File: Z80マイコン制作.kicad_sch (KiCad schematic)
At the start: 108 parts, among them M1 LED, SW1 SW_DIP_x08, SW2 SW_DIP_x08, SW3 SW_DIP_x08, SW4 SW_Push, SW5 SW_Push, SW6 SW_DIP_x01, SW7 SW_DIP_x08, U1 Z80CPU, U10 74HCT244, U11 74HCT244, U12 74HCT244, U13 74HCT244, U2 Z8420, U3 CY7C199, U4 74HCT244, U5 74HCT244, U6 74HCT244, U7 74HCT244, U8 74LS06N, U9 74LS06N, Y1 CXO_DIP8

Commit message: 回路図を作りました。まだ確認してません
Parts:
- removed RN4: 4.7k, Resistor_THT:R_Array_SIP9, symbol Device:R_Network08
- removed U8, U9: 74LS06N, Package_DIP:DIP-14_W7.62mm_Socket, symbol 74xx:74LS06N
- added C2, C3: 0.01u, Capacitor_THT:CP_Radial_D5.0mm_P2.00mm, symbol Device:C
- added J0, J1: Conn_01x08_Pin, Connector_PinHeader_2.54mm:PinHeader_1x08_P2.54mm_Vertical, symbol Connector:Conn_01x08_Pin
- added R39: 10k, Resistor_THT:R_Axial_DIN0204_L3.6mm_D1.6mm_P7.62mm_Horizontal, symbol Device:R
- added RN0, RN1, RN2, RN3, RN6: 4.7k, Resistor_THT:R_Array_SIP9, symbol Device:R_Network08
- added RV0: R_Potentiometer, Potentiometer_THT:Potentiometer_ACP_CA9-H5_Horizontal, symbol Device:R_Potentiometer
- added SW7: SW_Slide_DPDT, Button_Switch_THT:SW_E-Switch_EG1271_SPDT, symbol Switch:SW_Slide_DPDT
- added U13: NE555P, Package_DIP:DIP-8_W7.62mm, symbol Timer:NE555P
- A0: renamed from D7; footprint (none) -> LED_THT:LED_D3.0mm
- A1: renamed from D8; footprint (none) -> LED_THT:LED_D3.0mm
- A10: renamed from D17; footprint (none) -> LED_THT:LED_D3.0mm
- A11: renamed from D18; footprint (none) -> LED_THT:LED_D3.0mm
- A12: renamed from D21; footprint (none) -> LED_THT:LED_D3.0mm
- A13: renamed from D22; footprint (none) -> LED_THT:LED_D3.0mm
- A14: renamed from D23; footprint (none) -> LED_THT:LED_D3.0mm
- A2: renamed from D9; footprint (none) -> LED_THT:LED_D3.0mm
- A3: renamed from D10; footprint (none) -> LED_THT:LED_D3.0mm
- A4: renamed from D11; footprint (none) -> LED_THT:LED_D3.0mm
- A5: renamed from D12; footprint (none) -> LED_THT:LED_D3.0mm
- A6: renamed from D13; footprint (none) -> LED_THT:LED_D3.0mm
- A7: renamed from D14; footprint (none) -> LED_THT:LED_D3.0mm
- A8: renamed from D15; footprint (none) -> LED_THT:LED_D3.0mm
- A9: renamed from D16; footprint (none) -> LED_THT:LED_D3.0mm
- C1: renamed from C2; value 10u -> 100u
- CLK0: renamed from CLK; footprint (none) -> LED_THT:LED_D3.0mm
- D0: renamed from D25; footprint (none) -> LED_THT:LED_D3.0mm
- D1: renamed from D26; footprint (none) -> LED_THT:LED_D3.0mm
- D2: renamed from D27; footprint (none) -> LED_THT:LED_D3.0mm
- D3: renamed from D28; footprint (none) -> LED_THT:LED_D3.0mm
- D4: renamed from D29; footprint (none) -> LED_THT:LED_D3.0mm
- D5: renamed from D30; footprint (none) -> LED_THT:LED_D3.0mm
- D6: renamed from D31; footprint (none) -> LED_THT:LED_D3.0mm
- D7: renamed from D32; footprint (none) -> LED_THT:LED_D3.0mm
- D8: renamed from D40; footprint (none) -> LED_THT:LED_D3.0mm
- IORQ0: renamed from IORQ; footprint (none) -> LED_THT:LED_D3.0mm
- M0: renamed from M1; footprint (none) -> LED_THT:LED_D3.0mm
- MREQ0: renamed from MREQ; footprint (none) -> LED_THT:LED_D3.0mm
- R0: renamed from R9; footprint (none) -> Resistor_THT:R_Axial_DIN0204_L3.6mm_D1.6mm_P7.62mm_Horizontal
- R1: renamed from R10; footprint (none) -> Resistor_THT:R_Axial_DIN0204_L3.6mm_D1.6mm_P7.62mm_Horizontal
- R10: renamed from R19; footprint (none) -> Resistor_THT:R_Axial_DIN0204_L3.6mm_D1.6mm_P7.62mm_Horizontal
- R11: renamed from R20; footprint (none) -> Resistor_THT:R_Axial_DIN0204_L3.6mm_D1.6mm_P7.62mm_Horizontal
- R12: renamed from R21; footprint (none) -> Resistor_THT:R_Axial_DIN0204_L3.6mm_D1.6mm_P7.62mm_Horizontal
- R13: renamed from R22; footprint (none) -> Resistor_THT:R_Axial_DIN0204_L3.6mm_D1.6mm_P7.62mm_Horizontal
- R14: renamed from R23; footprint (none) -> Resistor_THT:R_Axial_DIN0204_L3.6mm_D1.6mm_P7.62mm_Horizontal
- R15: renamed from R25; footprint (none) -> Resistor_THT:R_Axial_DIN0204_L3.6mm_D1.6mm_P7.62mm_Horizontal
- R16: renamed from R26; footprint (none) -> Resistor_THT:R_Axial_DIN0204_L3.6mm_D1.6mm_P7.62mm_Horizontal
- R17: renamed from R27; footprint (none) -> Resistor_THT:R_Axial_DIN0204_L3.6mm_D1.6mm_P7.62mm_Horizontal
- R18: renamed from R28; footprint (none) -> Resistor_THT:R_Axial_DIN0204_L3.6mm_D1.6mm_P7.62mm_Horizontal
- R19: renamed from R29; footprint (none) -> Resistor_THT:R_Axial_DIN0204_L3.6mm_D1.6mm_P7.62mm_Horizontal
- R2: renamed from R11; footprint (none) -> Resistor_THT:R_Axial_DIN0204_L3.6mm_D1.6mm_P7.62mm_Horizontal
- R20: renamed from R30; footprint (none) -> Resistor_THT:R_Axial_DIN0204_L3.6mm_D1.6mm_P7.62mm_Horizontal
- R21: renamed from R31; footprint (none) -> Resistor_THT:R_Axial_DIN0204_L3.6mm_D1.6mm_P7.62mm_Horizontal
- R22: renamed from R32; footprint (none) -> Resistor_THT:R_Axial_DIN0204_L3.6mm_D1.6mm_P7.62mm_Horizontal
- R23: renamed from R33; footprint (none) -> Resistor_THT:R_Axial_DIN0204_L3.6mm_D1.6mm_P7.62mm_Horizontal
- R24: renamed from R34; footprint (none) -> Resistor_THT:R_Axial_DIN0204_L3.6mm_D1.6mm_P7.62mm_Horizontal
- R25: renamed from R35; footprint (none) -> Resistor_THT:R_Axial_DIN0204_L3.6mm_D1.6mm_P7.62mm_Horizontal
- R26: renamed from R36; footprint (none) -> Resistor_THT:R_Axial_DIN0204_L3.6mm_D1.6mm_P7.62mm_Horizontal
- R27: renamed from R37; footprint (none) -> Resistor_THT:R_Axial_DIN0204_L3.6mm_D1.6mm_P7.62mm_Horizontal
- R28: renamed from R38; footprint (none) -> Resistor_THT:R_Axial_DIN0204_L3.6mm_D1.6mm_P7.62mm_Horizontal
- R29: renamed from R39; footprint (none) -> Resistor_THT:R_Axial_DIN0204_L3.6mm_D1.6mm_P7.62mm_Horizontal
- R3: renamed from R12; footprint (none) -> Resistor_THT:R_Axial_DIN0204_L3.6mm_D1.6mm_P7.62mm_Horizontal
- R30: renamed from R40; footprint (none) -> Resistor_THT:R_Axial_DIN0204_L3.6mm_D1.6mm_P7.62mm_Horizontal
- R31: renamed from R8; footprint (none) -> Resistor_THT:R_Axial_DIN0204_L3.6mm_D1.6mm_P7.62mm_Horizontal
- R4: renamed from R13; footprint (none) -> Resistor_THT:R_Axial_DIN0204_L3.6mm_D1.6mm_P7.62mm_Horizontal
- R5: renamed from R14; footprint (none) -> Resistor_THT:R_Axial_DIN0204_L3.6mm_D1.6mm_P7.62mm_Horizontal
- R6: renamed from R15; footprint (none) -> Resistor_THT:R_Axial_DIN0204_L3.6mm_D1.6mm_P7.62mm_Horizontal
- R7: renamed from R16; footprint (none) -> Resistor_THT:R_Axial_DIN0204_L3.6mm_D1.6mm_P7.62mm_Horizontal
- R8: renamed from R17; footprint (none) -> Resistor_THT:R_Axial_DIN0204_L3.6mm_D1.6mm_P7.62mm_Horizontal
- R9: renamed from R18; footprint (none) -> Resistor_THT:R_Axial_DIN0204_L3.6mm_D1.6mm_P7.62mm_Horizontal
- RD0: renamed from RD; footprint (none) -> LED_THT:LED_D3.0mm
- WAIT0: renamed from WAIT; footprint (none) -> LED_THT:LED_D3.0mm
- WR0: renamed from WR; footprint (none) -> LED_THT:LED_D3.0mm
- renumbered SW2 to A0-A7, SW7 to A8-A14, C1 to C0, SW3 to D0-D7, SW1 to I0-I7, D1 to O0, D2 to O1, D3 to O2, D4 to O3, D5 to O4, D6 to O5, D19 to O6, D20 to O7, R3 to R32, R4 to R33, R5 to R34, R7 to R35, R6 to R36, R1 to R37, R2 to R38, RN3 to RN4, RN1 to RN5, RN5 to RN7, RN2 to RN8, SW5 to SW0, SW6 to SW1, TP1 to TP0, TP2 to TP1, U7 to U0, U10 to U1, U6 to U10, U12 to U2, U13 to U3, U1 to U4, U2 to U5, U3 to U6, U4 to U8, U5 to U9, SW4 to WRITE0, Y1 to Y0
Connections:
- net GND: now also A0-A7.1, A0-A7.2, A0-A7.3, A0-A7.4, A0-A7.5, A0-A7.6, A0-A7.7, A0-A7.8, O0.1 (K), O1.1 (K), O2.1 (K), O3.1 (K), O4.1 (K), O5.1 (K), O6.1 (K), O7.1 (K), RN5.2 (R1), RN5.3 (R2), RN5.4 (R3), RN5.5 (R4), RN5.6 (R5), RN5.7 (R6), RN5.8 (R7), RN5.9 (R8), U11.11 (2A3), U11.13 (2A2), U11.15 (2A1), U11.17 (2A0), U11.2 (1A0), U11.4 (1A1), U11.6 (1A2), U11.8 (1A3), SW7.5 (B); no longer Y0.4 (GND)
- net VCC: now also RN8.1 (common), R39.1, RN0.1 (common), RN1.1 (common), RN2.1 (common), RN3.1 (common), RN6.1 (common), U13.4 (R), U13.8 (VCC); no longer D0-D7.6, RN8.4 (R3), U8.15 (2A1)
- net at I0-I7.1, RN7.2 (R1), U5.15 (PA0): now also J1.8 (Pin_8)
- net at I0-I7.2, RN7.3 (R2), U5.14 (PA1): now also J1.7 (Pin_7)
- net at I0-I7.3, RN7.4 (R3), U5.13 (PA2): now also J1.6 (Pin_6)
- net at I0-I7.4, RN7.5 (R4), U5.12 (PA3): now also J1.5 (Pin_5)
- net at I0-I7.5, RN7.6 (R5), U5.10 (PA4): now also J1.4 (Pin_4)
- net at I0-I7.6, RN7.7 (R6), U5.9 (PA5): now also J1.3 (Pin_3)
- net at I0-I7.7, RN7.8 (R7), U5.8 (PA6): now also J1.2 (Pin_2)
- net at I0-I7.8, RN7.9 (R8), U5.7 (PA7): now also J1.1 (Pin_1)
- net at U10.1 (1OE), U10.19 (2OE), U11.1 (1OE)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: now also RN0.9 (R8)
- net at U10.14 (1Y2), U3.15 (2A1), U4.19 (~{MREQ})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: now also RN0.7 (R6)
- net at U10.16 (1Y1), U3.17 (2A0), U4.22 (~{WR})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: now also RN0.6 (R5)
- net at U10.18 (1Y0), U3.8 (1A3), U4.21 (~{RD})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: now also RN0.5 (R4)
- net at O3.2 (A): now also U5.31 (PB4), J0.4 (Pin_4), RN6.6 (R5)
- net at U1.8 (1A3), U4.1 (A11), U6.7 (A11)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: now also RN2.5 (R4)
- net at U1.6 (1A2), U4.40 (A10), U6.6 (A10)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: now also RN2.4 (R3)
- net at U1.4 (1A1), U4.39 (A9), U6.5 (A9)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: now also RN2.3 (R2)
- net at U1.2 (1A0), U4.38 (A8), U6.4 (A8)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: now also RN2.2 (R1)
- net at U1.17 (2A0), U4.2 (A12), U6.8 (A12)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: now also RN2.6 (R5)
- net at U1.15 (2A1), U4.3 (A13), U6.9 (A13)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: now also RN2.7 (R6)
- net at U1.13 (2A2), U4.4 (A14), U6.10 (A14)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: now also RN2.8 (R7)
- net at U2.8 (1A3), U4.8 (D3), U5.40 (D3)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: now also RN1.5 (R4)
- net at U2.6 (1A2), U4.12 (D2), U5.1 (D2)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: now also RN1.4 (R3)
- net at U2.4 (1A1), U4.15 (D1), U5.20 (D1)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: now also RN1.3 (R2)
- net at U2.2 (1A0), U4.14 (D0), U5.19 (D0)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: now also RN1.2 (R1)
- net at U2.17 (2A0), U4.7 (D4), U5.39 (D4)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: now also RN1.6 (R5)
- net at U2.15 (2A1), U4.9 (D5), U5.38 (D5)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: now also RN1.7 (R6)
- net at U2.13 (2A2), U4.10 (D6), U5.3 (D6)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: now also RN1.8 (R7)
- net at U2.11 (2A3), U4.13 (D7), U5.2 (D7)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: now also RN1.9 (R8)
- net at O4.2 (A): now also U5.30 (PB3), J0.5 (Pin_5), RN6.5 (R4)
- net at O5.2 (A): now also U5.29 (PB2), J0.6 (Pin_6), RN6.4 (R3)
- net at U5.27 (PB0): now also O7.2 (A), J0.8 (Pin_8), RN6.2 (R1)
- net at O0.2 (A): now also U5.34 (PB7), J0.1 (Pin_1), RN6.9 (R8)
- net at U0.11 (2A3), U11.9 (2Y3), U4.37 (A7)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: now also RN3.9 (R8)
- net at U0.13 (2A2), U11.7 (2Y2), U4.36 (A6)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: now also RN3.8 (R7)
- net at U0.15 (2A1), U11.5 (2Y1), U4.35 (A5)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: now also RN3.7 (R6)
- net at U0.17 (2A0), U11.3 (2Y0), U4.34 (A4)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: now also RN3.6 (R5)
- net at U0.2 (1A0), U11.18 (1Y0), U4.30 (A0)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: now also RN3.2 (R1)
- net at U0.4 (1A1), U11.16 (1Y1), U4.31 (A1)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: now also RN3.3 (R2)
- net at U0.6 (1A2), U11.14 (1Y2), U4.32 (A2)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: now also RN3.4 (R3)
- net at U0.8 (1A3), U11.12 (1Y3), U4.33 (A3)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: now also RN3.5 (R4)
- net at U3.2 (1A0), U4.6 (~{CLK}), U5.25 (CLK): now also RN0.2 (R1), SW7.2 (B); no longer R35.1, Y0.5 (OUT)
- net at U5.33 (PB6): now also O1.2 (A), J0.2 (Pin_2), RN6.8 (R7)
- net at U5.28 (PB1): now also O6.2 (A), J0.7 (Pin_7), RN6.3 (R2)
- net at O2.2 (A): now also U5.32 (PB5), J0.3 (Pin_3), RN6.7 (R6)
- net at U3.13 (2A2), U4.20 (~{IORQ}), U5.36 (~{IORQ})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: now also RN0.8 (R7)
- net at U3.4 (1A1), U4.27 (~{M1}), U5.37 (~{M1}): now also RN0.3 (R2)
- net at R34.2, U3.6 (1A2), U4.17 (~{NMI})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: now also RN0.4 (R3)
- new net: C2.2, C3.2, U13.1 (GND)
- new net: C3.1, RV0.2, U13.2 (TR), U13.6 (THR)
- new net: SW7.3 (C), U13.3 (Q)
- new net: C2.1, SW7.4 (A), U13.5 (CV)
- new net: R39.2, RV0.3, U13.7 (DIS)
- new net: D0-D7.6, RN8.4 (R3), U8.15 (2A1)
- new net: R35.1, SW7.1 (A), Y0.5 (OUT)
- new net: SW7.6 (C), Y0.4 (GND)
- no-connect marks 31 -> 27
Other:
- moved on the sheet: A0, A0-A7, A1, A10, A11, A12, A13, A14, A2, A3, A4, A5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

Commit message: 基盤確認済み、PCBに入りました
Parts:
- added R40: 4.7k, Resistor_THT:R_Axial_DIN0204_L3.6mm_D1.6mm_P7.62mm_Horizontal, symbol Device:R
- added U7: 74HCT244, Package_DIP:DIP-20_W7.62mm_Socket, symbol 74xx:74HCT244
- renumbered D8 to BUSACK0, SW0 to RESET0
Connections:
- net GND: no longer A0-A7.1, A0-A7.2, A0-A7.3, A0-A7.4, A0-A7.5, A0-A7.6, A0-A7.7, A0-A7.8, RN5.2 (R1), RN5.3 (R2), RN5.4 (R3), RN5.5 (R4), RN5.6 (R5), RN5.7 (R6), RN5.8 (R7), RN5.9 (R8), U11.11 (2A3), U11.13 (2A2), U11.15 (2A1), U11.17 (2A0), U11.2 (1A0), U11.4 (1A1), U11.6 (1A2), U11.8 (1A3)
- net VCC: now also R40.1
- net at J0.4 (Pin_4), O3.2 (A), RN6.6 (R5): now also U7.3 (2Y0); no longer U5.31 (PB4)
- net at J0.1 (Pin_1), O0.2 (A), RN6.9 (R8): now also U7.9 (2Y3); no longer U5.34 (PB7)
- net at J0.2 (Pin_2), O1.2 (A), RN6.8 (R7): now also U7.7 (2Y2); no longer U5.33 (PB6)
- net at J0.3 (Pin_3), O2.2 (A), RN6.7 (R6): now also U7.5 (2Y1); no longer U5.32 (PB5)
- net at J0.5 (Pin_5), O4.2 (A), RN6.5 (R4): now also U7.12 (1Y3); no longer U5.30 (PB3)
- net at J0.6 (Pin_6), O5.2 (A), RN6.4 (R3): now also U7.14 (1Y2); no longer U5.29 (PB2)
- net at J0.7 (Pin_7), O6.2 (A), RN6.3 (R2): now also U7.16 (1Y1); no longer U5.28 (PB1)
- net at J0.8 (Pin_8), O7.2 (A), RN6.2 (R1): now also U7.18 (1Y0); no longer U5.27 (PB0)
- new net: A0-A7.1, RN5.2 (R1), U11.2 (1A0)
- new net: A0-A7.2, RN5.3 (R2), U11.4 (1A1)
- new net: A0-A7.3, RN5.4 (R3), U11.6 (1A2)
- new net: A0-A7.4, RN5.5 (R4), U11.8 (1A3)
- new net: A0-A7.5, RN5.6 (R5), U11.17 (2A0)
- new net: A0-A7.6, RN5.7 (R6), U11.15 (2A1)
- new net: A0-A7.7, RN5.8 (R7), U11.13 (2A2)
- new net: A0-A7.8, RN5.9 (R8), U11.11 (2A3)
- new net: R40.2, U7.1 (1OE), U7.19 (2OE)
- new net: U5.34 (PB7), U7.11 (2A3)
- new net: U5.33 (PB6), U7.13 (2A2)
- new net: U5.32 (PB5), U7.15 (2A1)
- new net: U5.31 (PB4), U7.17 (2A0)
- new net: U5.27 (PB0), U7.2 (1A0)
- new net: U5.28 (PB1), U7.4 (1A1)
- new net: U5.29 (PB2), U7.6 (1A2)
- new net: U5.30 (PB3), U7.8 (1A3)
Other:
- moved on the sheet: D0-D7, I0-I7, J0, J1, O0, O1, O2, O3, O4, O5, O6, O7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

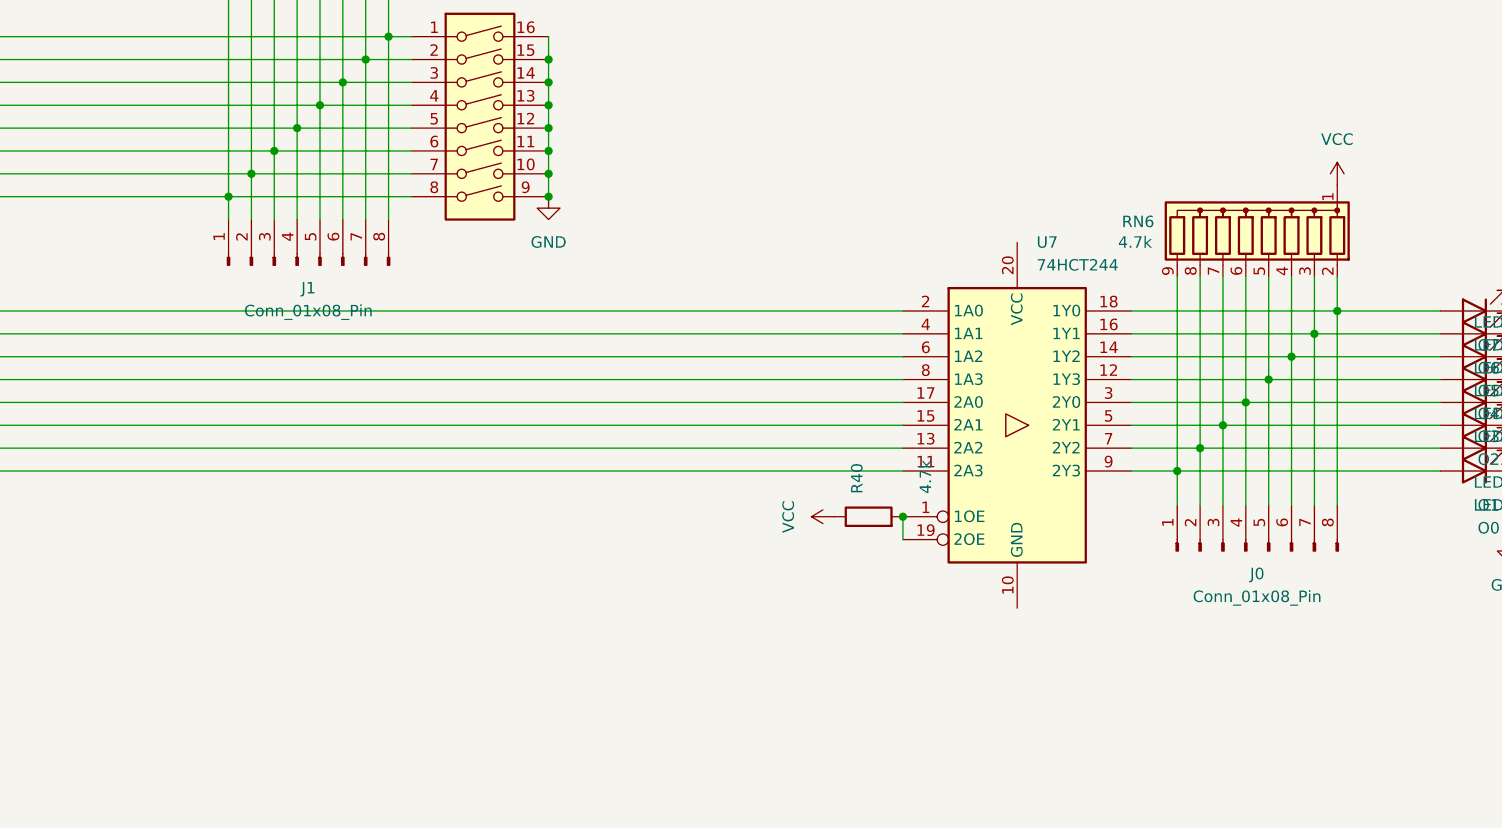
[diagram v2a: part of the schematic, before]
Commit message: 基盤のVCC,GND配線終わりました
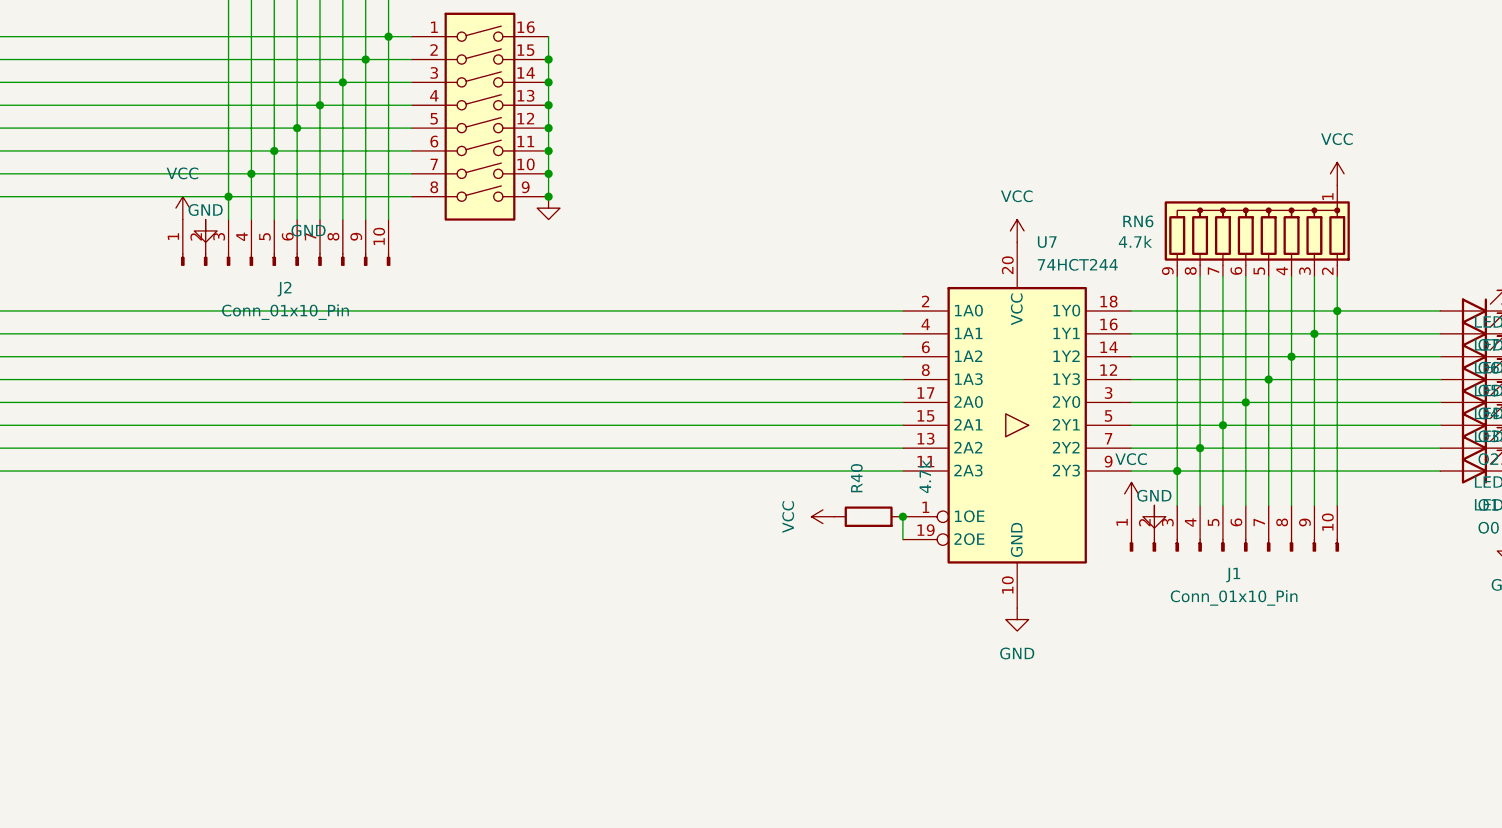
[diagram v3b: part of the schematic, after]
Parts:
- removed J0, J1: Conn_01x08_Pin, Connector_PinHeader_2.54mm:PinHeader_1x08_P2.54mm_Vertical, symbol Connector:Conn_01x08_Pin
- added J1, J2: Conn_01x10_Pin, Connector_PinHeader_2.54mm:PinHeader_1x10_P2.54mm_Vertical, symbol Connector:Conn_01x10_Pin
- A0-A7, A8-A14, D0-D7, I0-I7: footprint Package_DIP:CERDIP-16_W7.62mm_SideBrazed_Socket -> Package_DIP:DIP-16_W7.62mm_Socket
- U13: footprint Package_DIP:DIP-8_W7.62mm -> Package_DIP:DIP-8_W7.62mm_Socket
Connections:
- net GND: now also U7.10 (GND), J1.2 (Pin_2), J2.2 (Pin_2)
- net VCC: now also U7.20 (VCC), J1.1 (Pin_1), J2.1 (Pin_1)
- net at I0-I7.1, RN7.2 (R1), U5.15 (PA0): now also J2.10 (Pin_10)
- net at I0-I7.2, RN7.3 (R2), U5.14 (PA1): now also J2.9 (Pin_9)
- net at I0-I7.3, RN7.4 (R3), U5.13 (PA2): now also J2.8 (Pin_8)
- net at I0-I7.4, RN7.5 (R4), U5.12 (PA3): now also J2.7 (Pin_7)
- net at I0-I7.5, RN7.6 (R5), U5.10 (PA4): now also J2.6 (Pin_6)
- net at I0-I7.6, RN7.7 (R6), U5.9 (PA5): now also J2.5 (Pin_5)
- net at I0-I7.7, RN7.8 (R7), U5.8 (PA6): now also J2.4 (Pin_4)
- net at I0-I7.8, RN7.9 (R8), U5.7 (PA7): now also J2.3 (Pin_3)
- net at O3.2 (A), RN6.6 (R5), U7.3 (2Y0): now also J1.6 (Pin_6)
- net at O0.2 (A), RN6.9 (R8), U7.9 (2Y3): now also J1.3 (Pin_3)
- net at O1.2 (A), RN6.8 (R7), U7.7 (2Y2): now also J1.4 (Pin_4)
- net at O2.2 (A), RN6.7 (R6), U7.5 (2Y1): now also J1.5 (Pin_5)
- net at O4.2 (A), RN6.5 (R4), U7.12 (1Y3): now also J1.7 (Pin_7)
- net at O5.2 (A), RN6.4 (R3), U7.14 (1Y2): now also J1.8 (Pin_8)
- net at O6.2 (A), RN6.3 (R2), U7.16 (1Y1): now also J1.9 (Pin_9)
- net at O7.2 (A), RN6.2 (R1), U7.18 (1Y0): now also J1.10 (Pin_10)
